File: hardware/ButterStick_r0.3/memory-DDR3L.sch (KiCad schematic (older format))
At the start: 0 parts

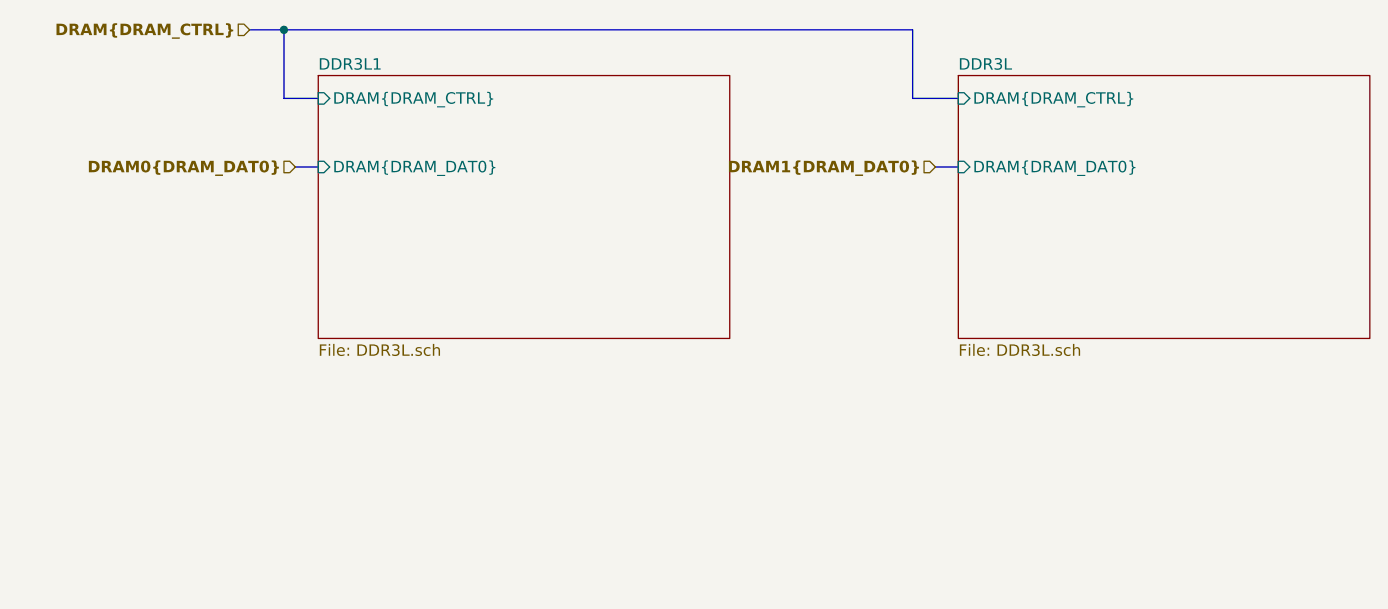
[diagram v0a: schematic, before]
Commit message: hw.r0_3: cleanup and additions
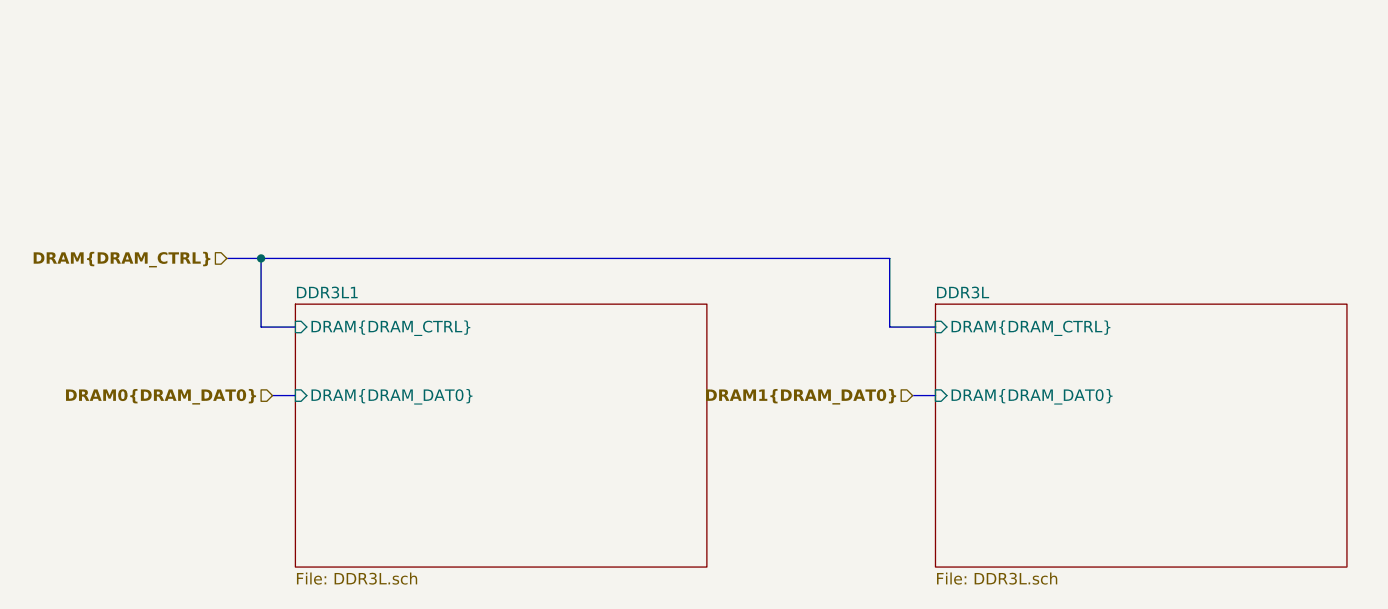
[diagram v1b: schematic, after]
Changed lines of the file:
@@
 $Descr A4 11693 8268
 encoding utf-8
-Sheet 4 16
+Sheet 16 20
 Title "ButterStick"
 Date "2019-06-14"
@@
 Comment9 ""
 $EndDescr
-Connection ~ 3650 1950
+Connection ~ 3550 2950
 Wire Bus Line
-	3500 1950 3650 1950
+	3400 2950 3550 2950
 Wire Bus Line
-	3650 1950 6400 1950
+	3550 2950 6300 2950
 Wire Bus Line
-	3650 2250 3650 1950
+	3550 3250 3550 2950
 Wire Bus Line
-	3700 2550 3800 2550
+	3600 3550 3700 3550
 Wire Bus Line
-	3800 2250 3650 2250
+	3700 3250 3550 3250
 Wire Bus Line
-	6400 1950 6400 2250
+	6300 2950 6300 3250
 Wire Bus Line
-	6400 2250 6600 2250
+	6300 3250 6500 3250
 Wire Bus Line
-	6500 2550 6600 2550
-Text HLabel 3500 1950 0    50   Input ~ 10
+	6400 3550 6500 3550
+Text HLabel 3400 2950 0    50   Input ~ 10
 DRAM{DRAM_CTRL}
-Text HLabel 3700 2550 0    50   Input ~ 10
+Text HLabel 3600 3550 0    50   Input ~ 10
 DRAM0{DRAM_DAT0}
-Text HLabel 6500 2550 0    50   Input ~ 10
+Text HLabel 6400 3550 0    50   Input ~ 10
 DRAM1{DRAM_DAT0}
 $Sheet
-S 6600 2150 1800 1150
+S 6500 3150 1800 1150
 U 5EB15CF3
 F0 "DDR3L" 50
 F1 "DDR3L.sch" 50
-F2 "DRAM{DRAM_DAT0}" I L 6600 2550 50
-F3 "DRAM{DRAM_CTRL}" I L 6600 2250 50
+F2 "DRAM{DRAM_DAT0}" I L 6500 3550 50
+F3 "DRAM{DRAM_CTRL}" I L 6500 3250 50
 $EndSheet
 $Sheet
-S 3800 2150 1800 1150
+S 3700 3150 1800 1150
 U 5EB207D6
 F0 "DDR3L1" 50
 F1 "DDR3L.sch" 50
-F2 "DRAM{DRAM_DAT0}" I L 3800 2550 50
-F3 "DRAM{DRAM_CTRL}" I L 3800 2250 50
+F2 "DRAM{DRAM_DAT0}" I L 3700 3550 50
+F3 "DRAM{DRAM_CTRL}" I L 3700 3250 50
 $EndSheet
 $EndSCHEMATC
